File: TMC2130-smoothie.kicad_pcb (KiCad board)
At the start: 4 copper layers, 38.1 x 156.2 mm, 286 parts, among them P1 CONN_01X04, P2 CONN_01X04, P3 CONN_01X04, P4 CONN_01X04, P5 CONN_01X26, P6 Vmot, U1 TMC2130, U2 TMC2130, U3 TMC2130, U4 TMC2130, U5 AP1117-3v3

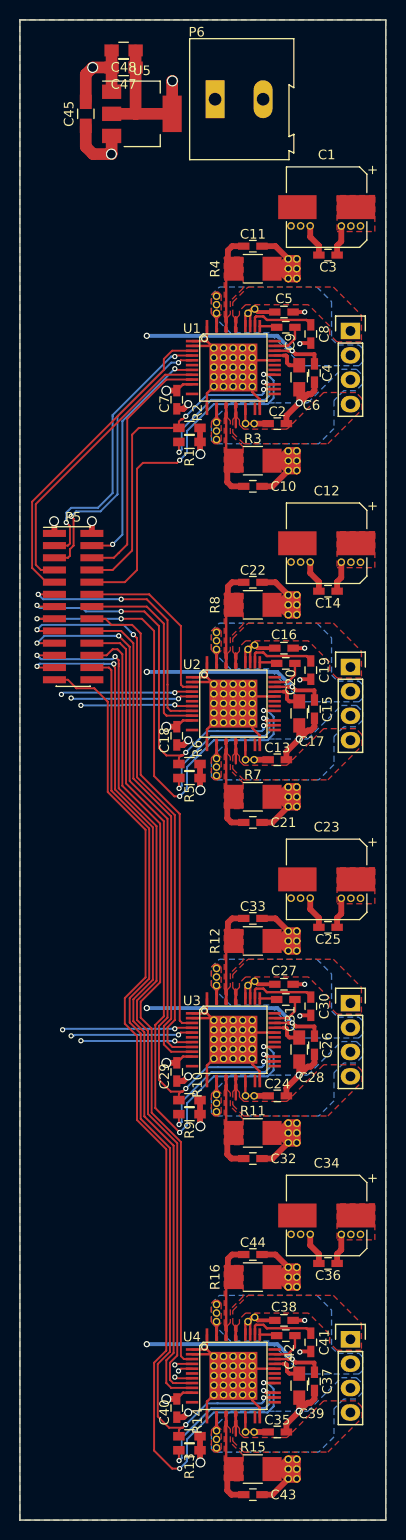
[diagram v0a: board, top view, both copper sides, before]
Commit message: Added gerbers
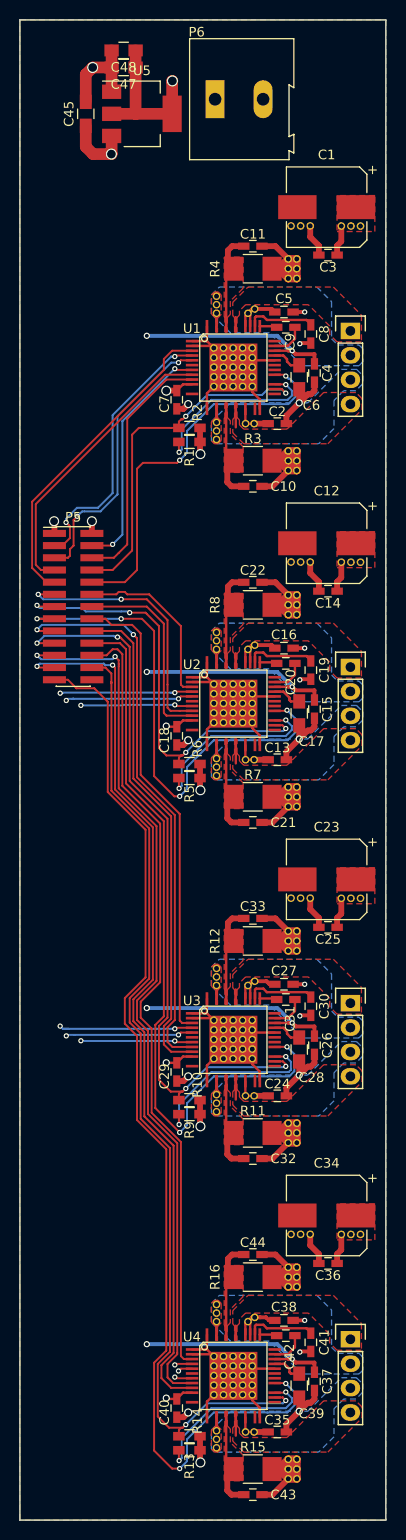
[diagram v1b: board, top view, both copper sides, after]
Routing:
- net M1_DIAG0: track 34.5 -> 36.9 mm
- net M3_DIAG0: track 74.4 -> 76.6 mm
- net M2_DIAG0: track 43.0 -> 45.1 mm
- net M2_EN: track 51.3 -> 53.3 mm
- net M1_EN: track 38.7 -> 40.7 mm
- net M4_DIAG0: track 99.8 -> 101.8 mm
- net M3_EN: track 75.3 -> 77.3 mm
- net SPI_MOSI: track 159.4 -> 161.3 mm
- net M4_EN: track 110.9 -> 112.7 mm
- net M4_DIAG1: track 17.3 -> 19.1 mm
- net M1_DIAG1: track 17.3 -> 19.1 mm
- net M3_DIAG1: track 17.3 -> 19.1 mm
- net M2_DIAG1: track 17.3 -> 19.1 mm
- net SPI_SCK: track 164.3 -> 165.9 mm
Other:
- net class Default: clearance 0.127 -> 0.1524; trace_width 0.127 -> 0.1524; via_dia 0.4572 -> 0.55; via_drill 0.254 -> 0.3
- rule trace_clearance: 0.127 -> 0.1524
- rule trace_min: 0.127 -> 0.1524
- rule via_min_size: 0.4572 -> 0.54991
